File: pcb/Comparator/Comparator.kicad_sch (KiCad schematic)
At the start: 17 parts, among them J1 Conn_01x04_Pin, J2 Conn_01x04_Pin, U1 LT1711xMS8

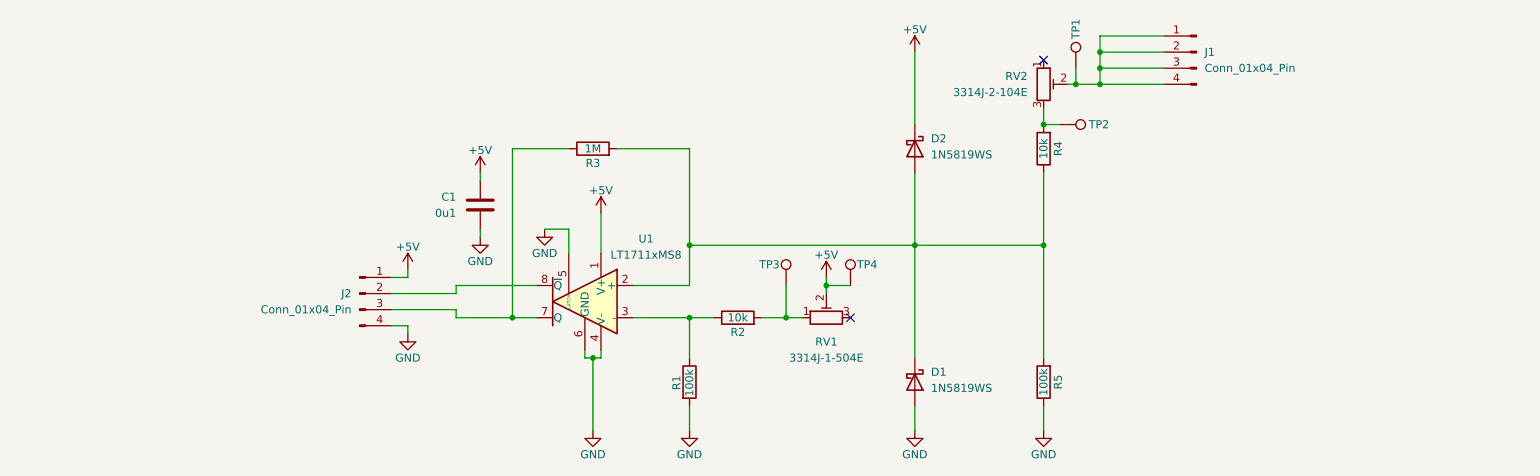
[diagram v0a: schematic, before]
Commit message: d
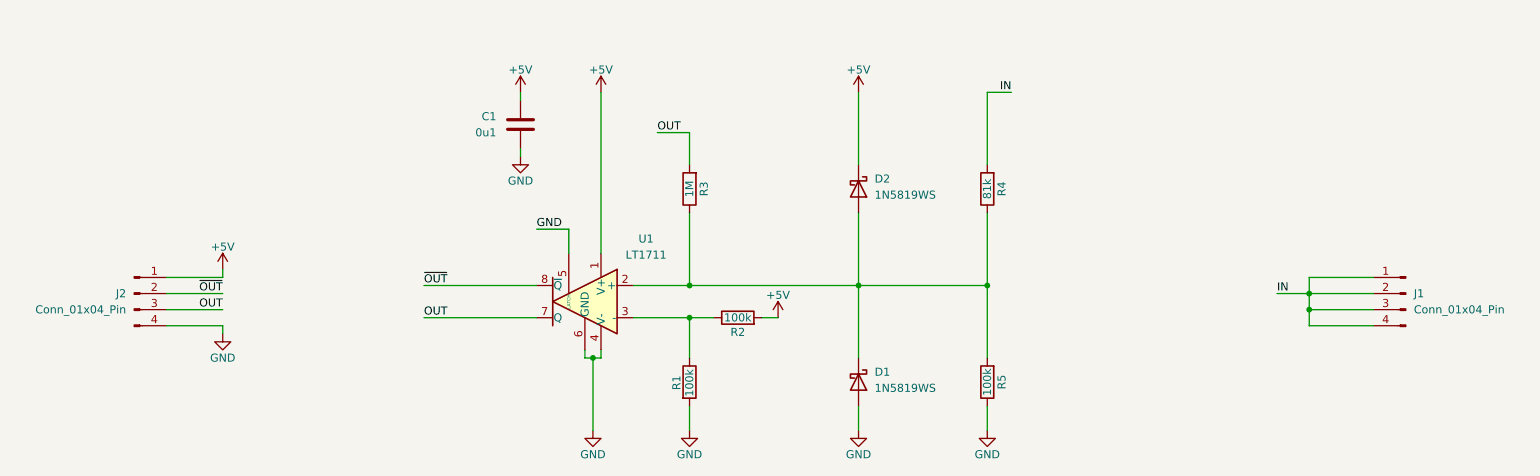
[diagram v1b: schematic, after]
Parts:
- removed RV1: 3314J-1-504E, Potentiometer_SMD:Potentiometer_Bourns_3314J_Vertical, symbol Device:R_Potentiometer_Trim
- removed RV2: 3314J-2-104E, Potentiometer_SMD:Potentiometer_Bourns_3314J_Vertical, symbol Device:R_Potentiometer_Trim
- removed TP1, TP2, TP3, TP4: TestPoint, TestPoint:TestPoint_Pad_D1.5mm, symbol Connector:TestPoint
- R2: value 10k -> 100k
- R4: value 10k -> 81k
- U1: value LT1711xMS8 -> LT1711
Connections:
- net +5V: now also R2.2
- net at D1.1 (K), D2.2 (A), R4.1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: now also R3.1; no longer R3.2
- net OUT: now reaches J2.3 (Pin_3), U1.7 (Q)
- net OUT: now also R3.2; no longer R3.1
- net ~{OUT}: now reaches J2.2 (Pin_2), U1.8 (~{Q})
- net IN: now reaches J1.1 (Pin_1), J1.2 (Pin_2), J1.3 (Pin_3), J1.4 (Pin_4)
- net IN: now also R4.2
- no-connect marks 2 -> 0
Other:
- moved on the sheet: C1, D1, D2, J1, J2, R3, R4, R5
